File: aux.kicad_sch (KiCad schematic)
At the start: 17 parts, among them J7 USB_C_Receptacle_USB2.0_16P, J86 Conn_01x02_Pin, Q81 Si2301CDS, Q82 AO3400A, U85 DAC80508xRTE

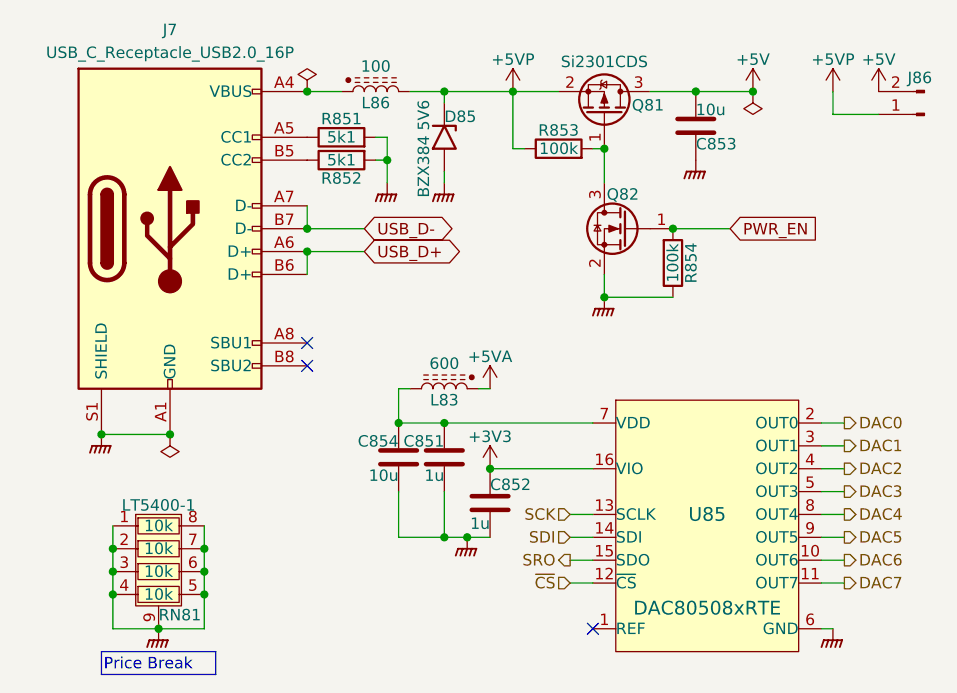
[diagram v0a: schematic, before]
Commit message: Most blocks there....
About to restore scan.
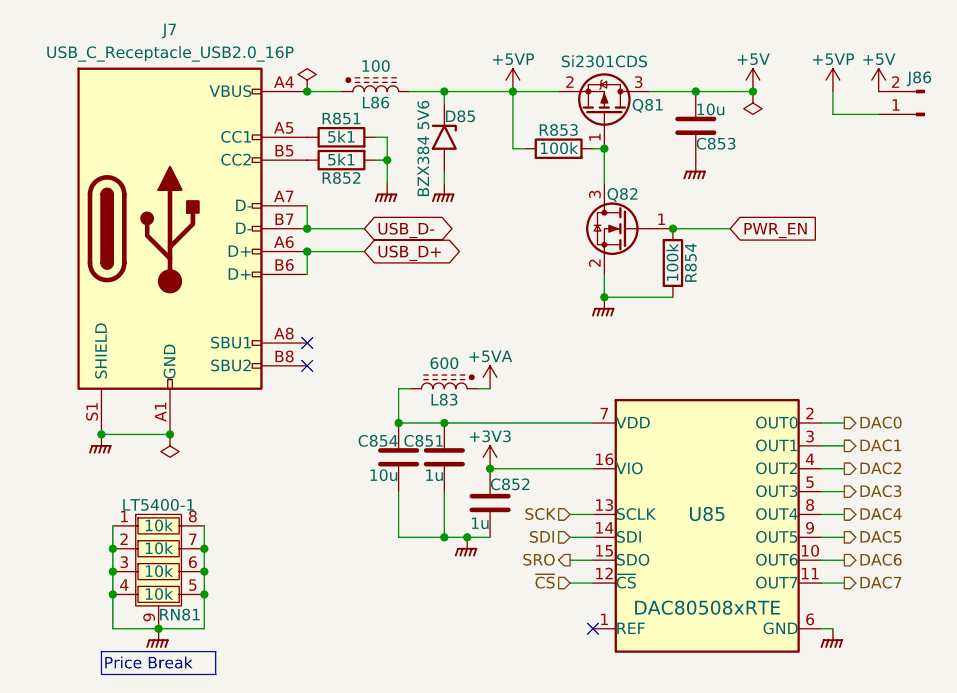
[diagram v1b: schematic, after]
